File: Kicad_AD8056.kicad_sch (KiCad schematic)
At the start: 4 parts, among them J1 Conn_Coaxial, U1 AD8056AR

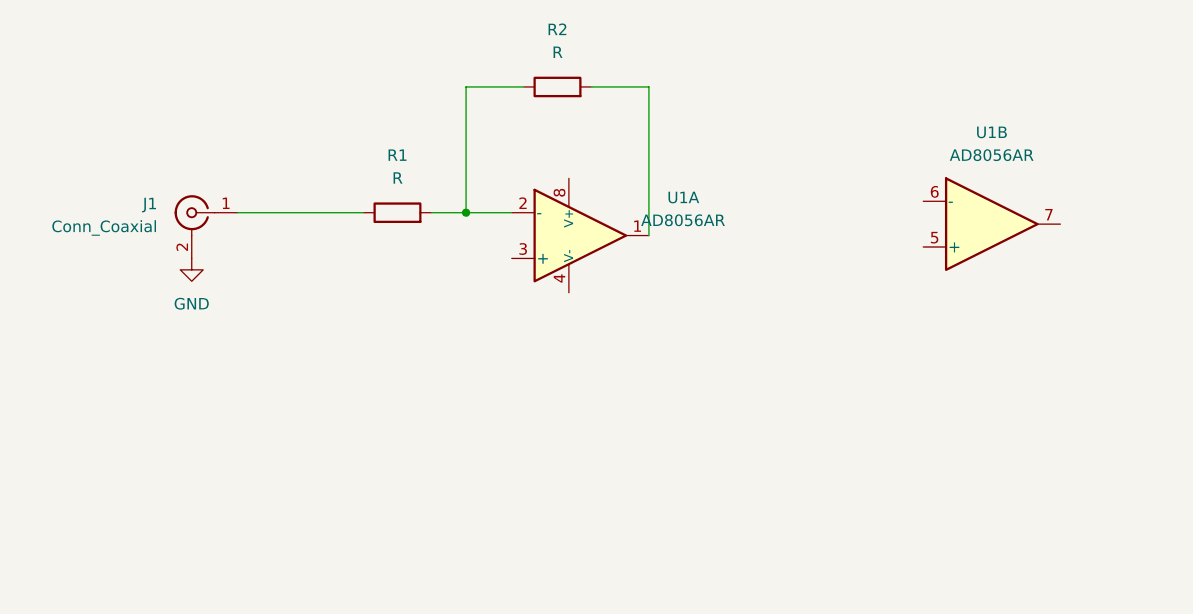
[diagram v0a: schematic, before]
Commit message: add new pcb
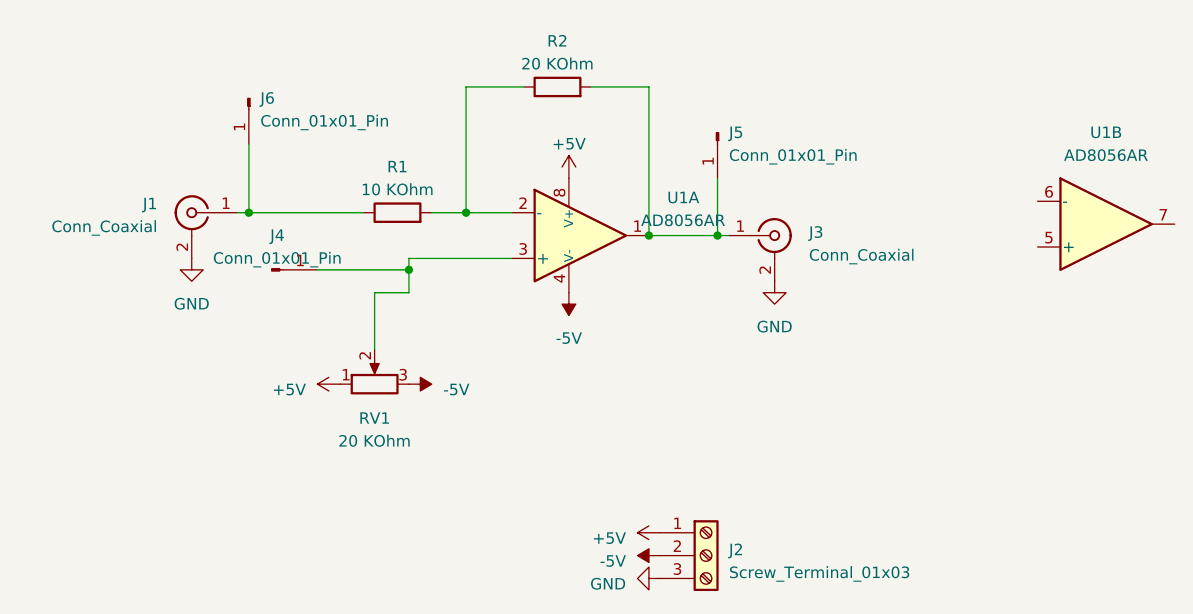
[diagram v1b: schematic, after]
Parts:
- added J2: Screw_Terminal_01x03, TerminalBlock:TerminalBlock_bornier-3_P5.08mm, symbol Connector:Screw_Terminal_01x03
- added J3: Conn_Coaxial, Connector_Coaxial:BNC_Amphenol_B6252HB-NPP3G-50_Horizontal, symbol Connector:Conn_Coaxial
- added J4, J5, J6: Conn_01x01_Pin, Connector_Pin:Pin_D1.0mm_L10.0mm, symbol Connector:Conn_01x01_Pin
- added RV1: 20 KOhm, Potentiometer_THT:Potentiometer_Alps_RK163_Single_Horizontal, symbol Device:R_Potentiometer
- R1: value R -> 10 KOhm; footprint (none) -> Resistor_SMD:R_0805_2012Metric
- R2: value R -> 20 KOhm; footprint (none) -> Resistor_SMD:R_0805_2012Metric
- U1: footprint Package_SO:SOIC-8-1EP_3.9x4.9mm_P1.27mm_EP2.29x3mm -> Package_SO:SSOP-8_3.9x5.05mm_P1.27mm
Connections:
- net GND: now also J2.3 (Pin_3), J3.2 (Ext)
- net at R2.2, U1.1: now also J3.1 (In), J5.1 (Pin_1)
- net at J1.1 (In), R1.1: now also J6.1 (Pin_1)
- net at U1.3 (+): now also J4.1 (Pin_1), RV1.2
- net -5V: now reaches U1.4 (V-)
- net -5V: now also J2.2 (Pin_2), RV1.3
- net +5V: now reaches U1.8 (V+)
- net +5V: now also J2.1 (Pin_1), RV1.1
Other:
- moved on the sheet: U1B
